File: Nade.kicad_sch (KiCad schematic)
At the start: 44 parts, among them J1 FTSH-107-01-L-DV-K, J2 Conn_01x03_Pin, J3 UART_IN, J4 BATT, J5 MEM2085-00-115-00-A_REV0.2, J6 Conn_01x02_Pin, J8 Buzzer, Q1 NMOS, Q2 NMOS, SW2 SW_SPDT, SW3 PTS526 SM15 SMTR2 LFS, U1 MP28160GC-Z, U2 INA213AIRSWR, U3 ADXL314WBCPZ-RL, U4 SSM6N7002KFU_LF

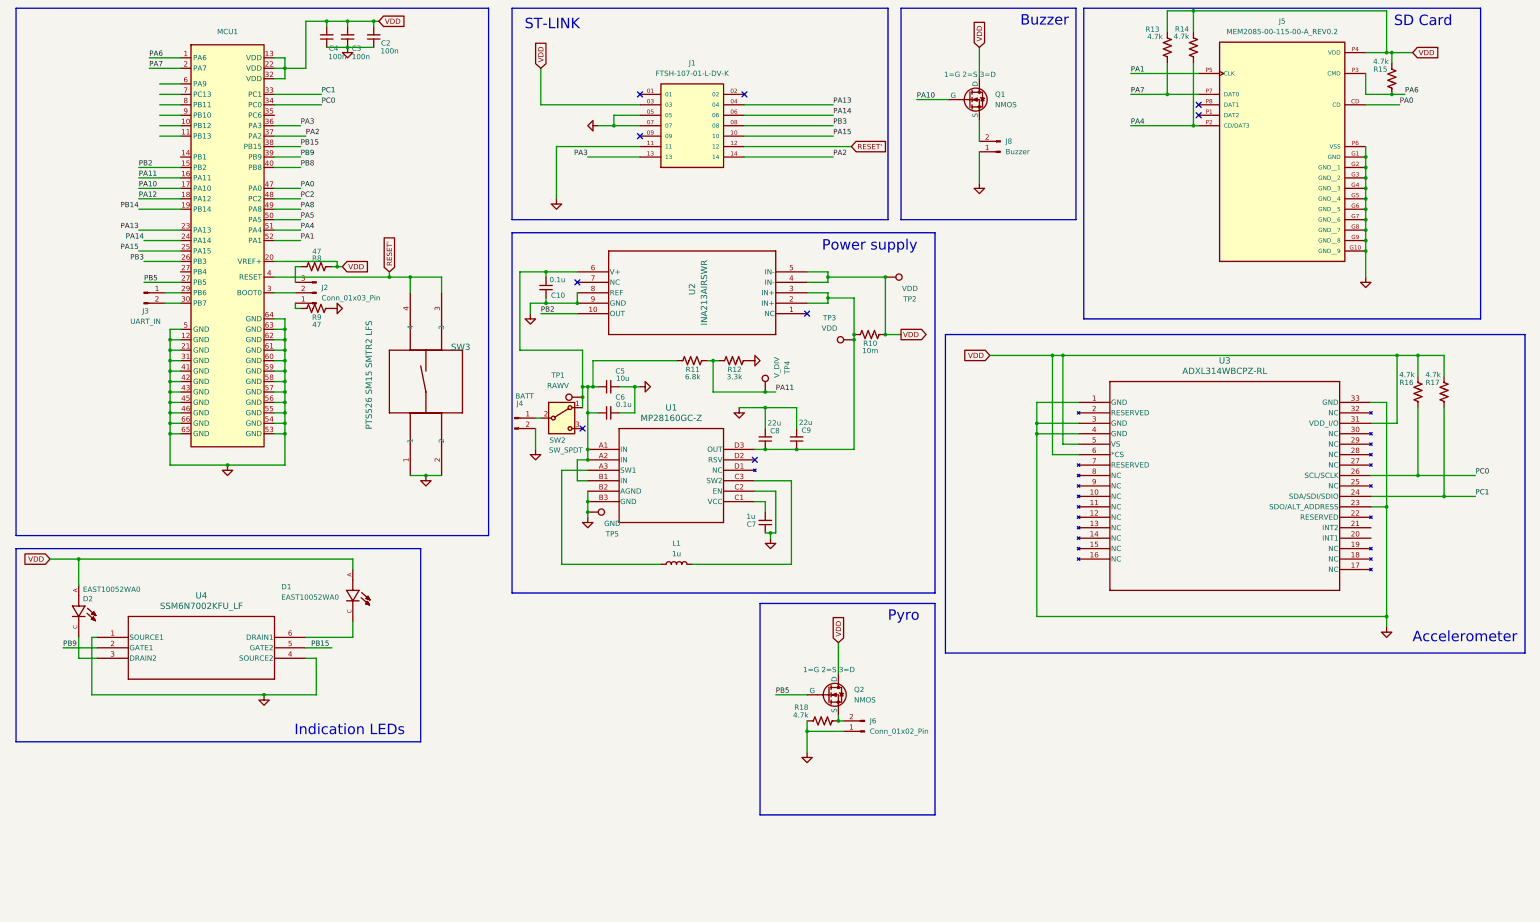
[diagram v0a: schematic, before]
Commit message: v2
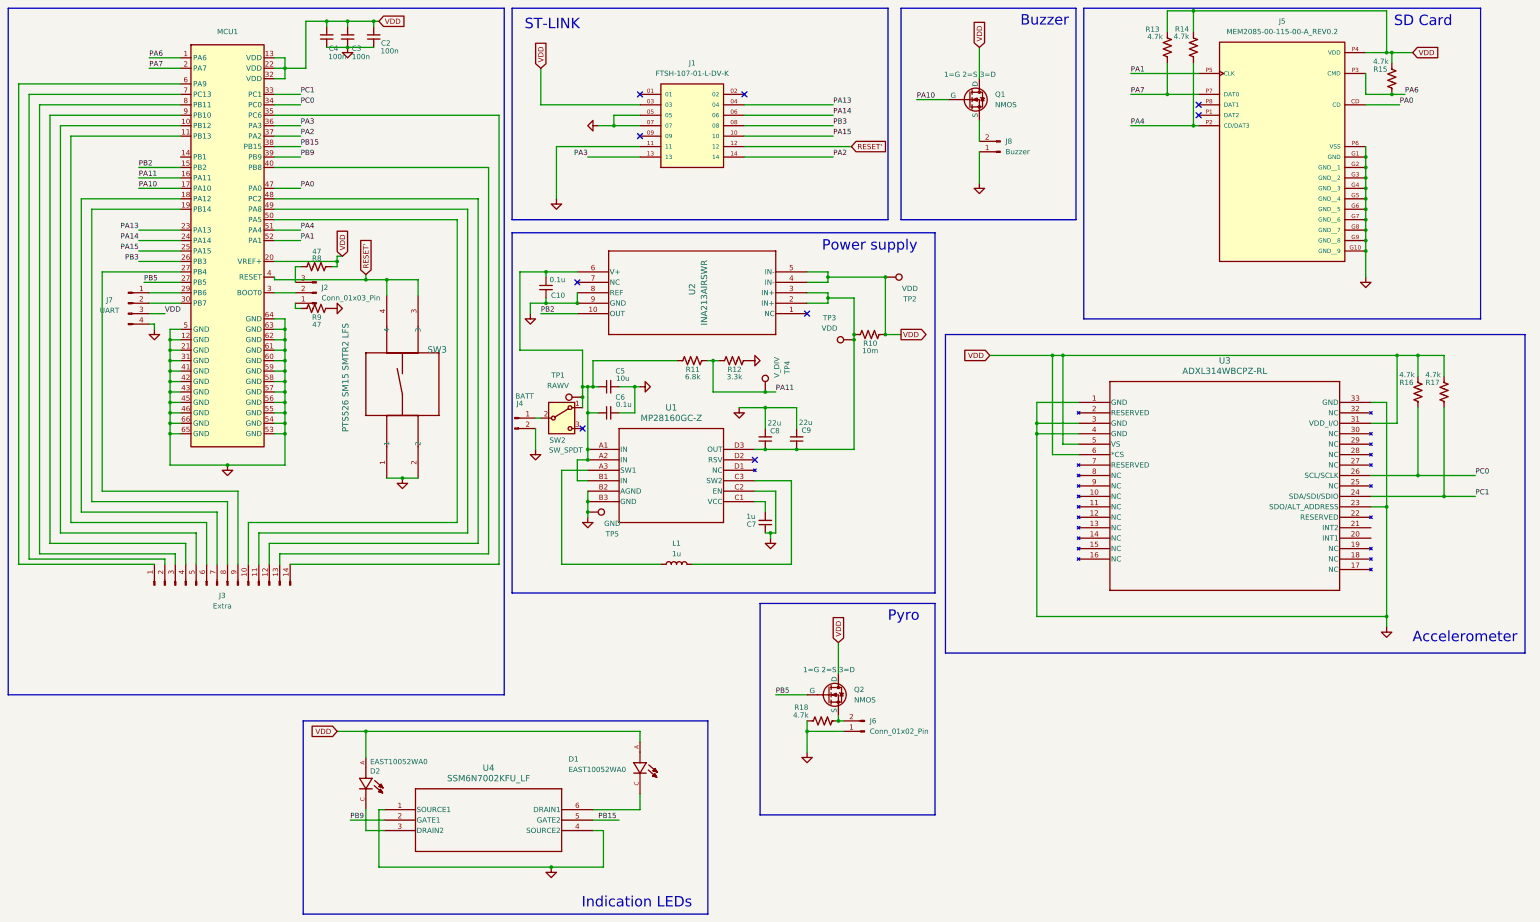
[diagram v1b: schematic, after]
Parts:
- removed J3: UART_IN, Connector_JST:JST_SH_BM02B-SRSS-TB_1x02-1MP_P1.00mm_Vertical, symbol Connector:Conn_01x02_Pin
- added J3: Extra, Connector_PinHeader_1.27mm:PinHeader_2x07_P1.27mm_Vertical_SMD, symbol Connector:Conn_01x14_Pin
- added J7: UART, Connector_JST:JST_SH_SM04B-SRSS-TB_1x04-1MP_P1.00mm_Horizontal, symbol Connector:Conn_01x04_Pin
- TP5: footprint TestPoint:TestPoint_Loop_D2.50mm_Drill1.85mm -> TestPoint:TestPoint_THTPad_2.0x2.0mm_Drill1.0mm
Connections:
- net GND: now also J7.4 (Pin_4)
- net VDD: now also J7.3 (Pin_3)
- net at MCU1.10 (PB12): now also J3.5 (Pin_5)
- net at MCU1.11 (PB13): now also J3.6 (Pin_6)
- net at MCU1.29 (PB6): now also J7.1 (Pin_1)
- net at MCU1.30 (PB7): now also J7.2 (Pin_2)
- net at MCU1.35 (PC6): now also J3.14 (Pin_14)
- net at MCU1.6 (PA9): now also J3.1 (Pin_1)
- net at MCU1.7 (PC13): now also J3.2 (Pin_2)
- net at MCU1.8 (PB11): now also J3.3 (Pin_3)
- net at MCU1.9 (PB10): now also J3.4 (Pin_4)
- net PA12: no longer names the net of MCU1.18 (PA12)
- net PA12: now also J3.7 (Pin_7)
- net PA5: no longer names the net of MCU1.50 (PA5)
- net PA5: now also J3.10 (Pin_10)
- net PA8: no longer names the net of MCU1.49 (PA8)
- net PA8: now also J3.11 (Pin_11)
- net PB14: no longer names the net of MCU1.19 (PB14)
- net PB14: now also J3.8 (Pin_8)
- net PB8: no longer names the net of MCU1.40 (PB8)
- net PB8: now also J3.13 (Pin_13)
- net PC2: no longer names the net of MCU1.48 (PC2)
- net PC2: now also J3.12 (Pin_12)
- new net: J3.9 (Pin_9), MCU1.27 (PB5)
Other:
- moved on the sheet: D1, D2, SW3, U4
